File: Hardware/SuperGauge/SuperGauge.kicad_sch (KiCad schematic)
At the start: 20 parts, among them J102 MainConn, Q602 MMBT3906, U103 ATmega16U2, U301 NCV1117ST50T3G

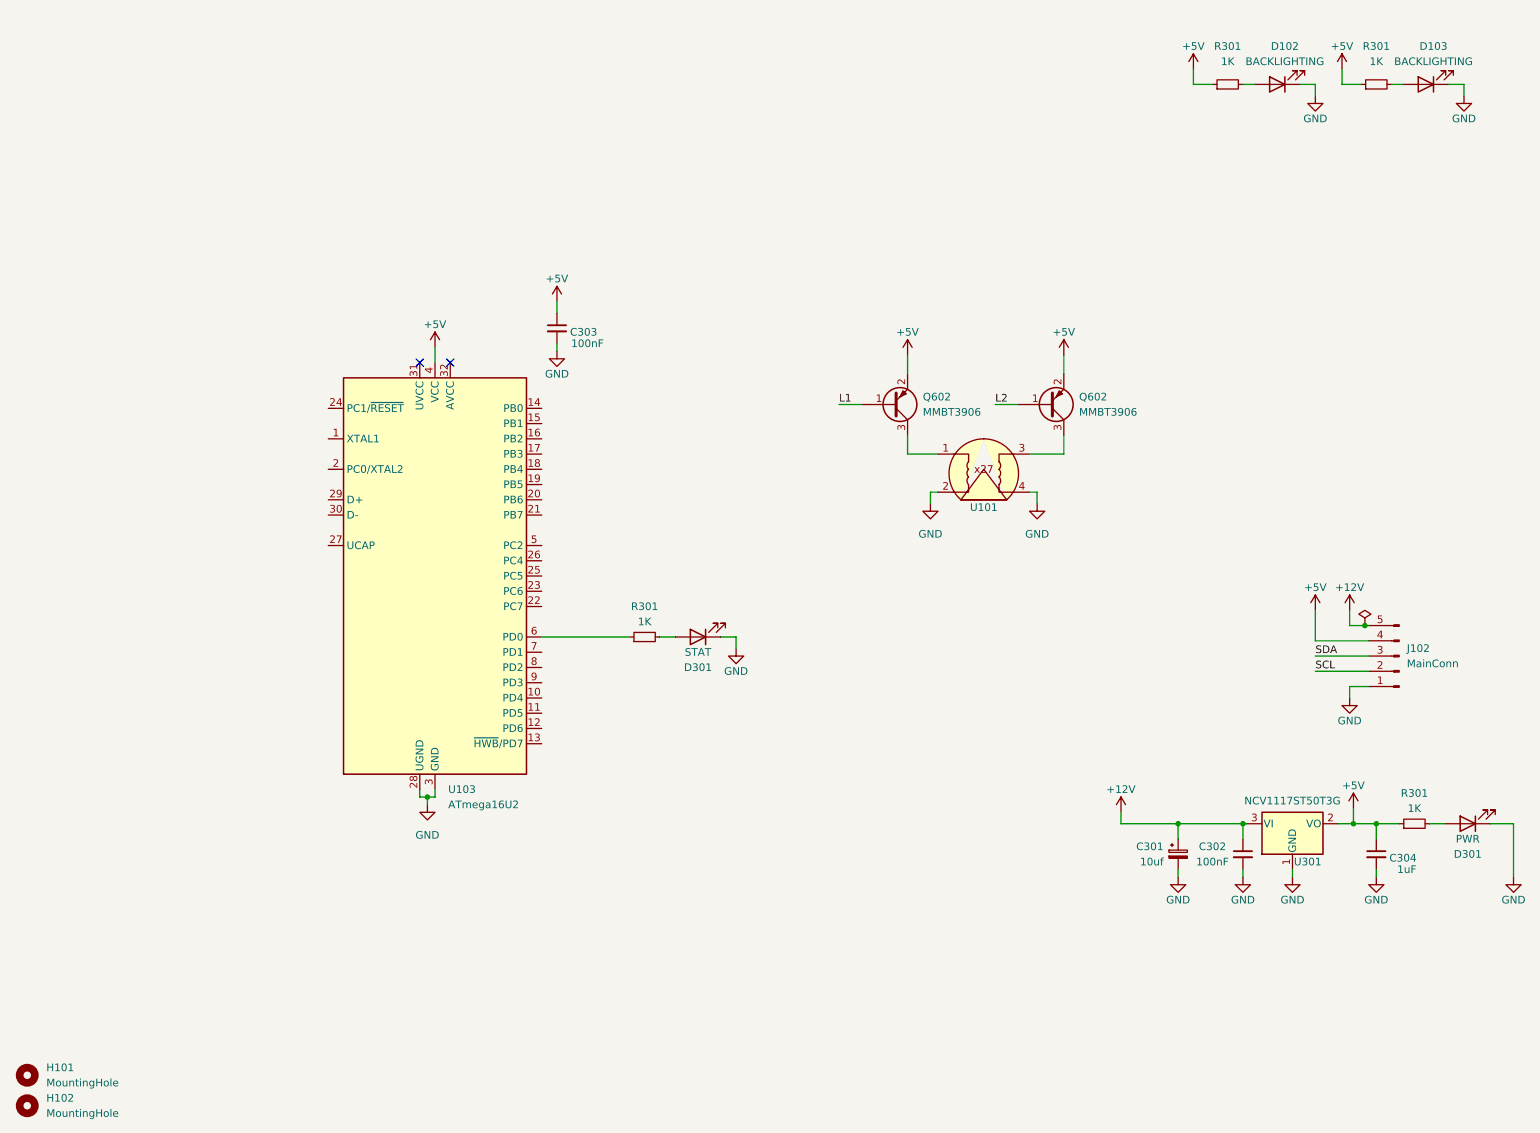
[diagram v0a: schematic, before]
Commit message: More PCB stuff
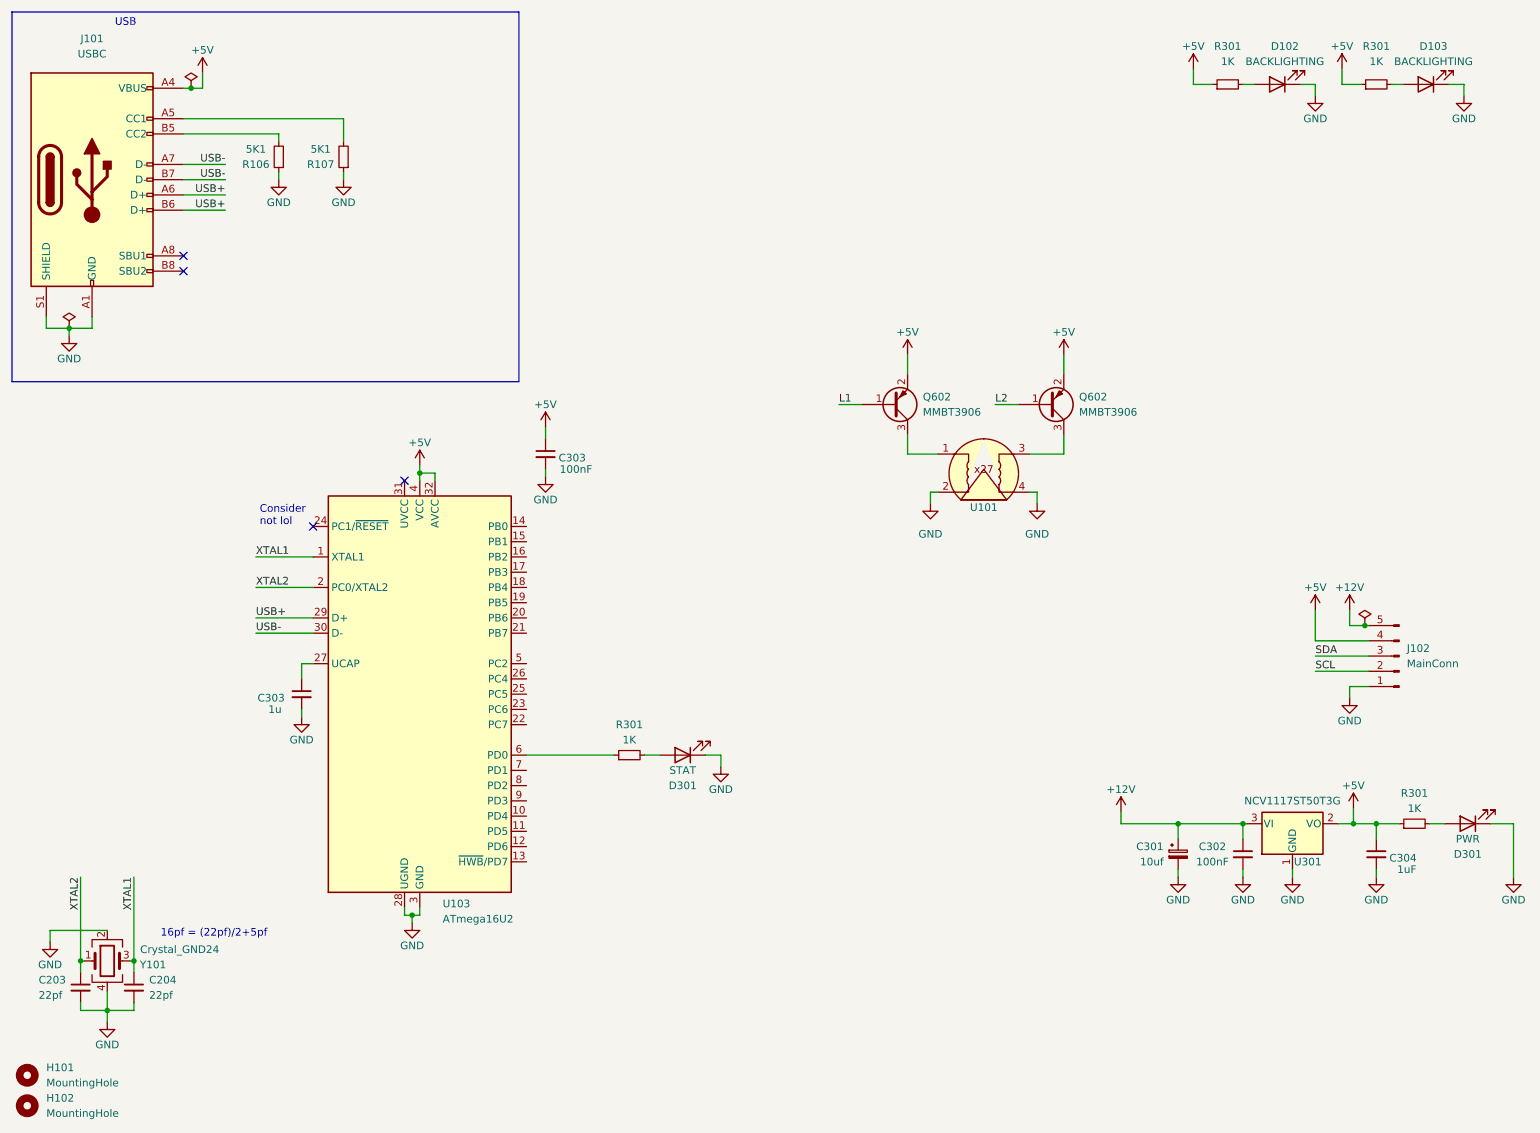
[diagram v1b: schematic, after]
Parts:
- added C203, C204: 22pf, Capacitor_SMD:C_0603_1608Metric, symbol Device:C_Small
- added C303: 1u, Capacitor_SMD:C_0805_2012Metric, symbol Device:C_Small
- added J101: USBC, Connector_USB:USB_C_Receptacle_XKB_U262-16XN-4BVC11, symbol Connector:USB_C_Receptacle_USB2.0
- added R106, R107: 5K1, Resistor_SMD:R_0805_2012Metric, symbol Device:R_Small
- added Y101: Crystal_GND24, Crystal:Crystal_SMD_3225-4Pin_3.2x2.5mm, symbol Device:Crystal_GND24
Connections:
- net +5V: now also U103.32 (AVCC), J101.A4 (VBUS), J101.A9 (VBUS), J101.B4 (VBUS), J101.B9 (VBUS)
- net GND: now also C203.2, C204.2, C303.2, J101.A1 (GND), J101.A12 (GND), J101.B1 (GND), J101.B12 (GND), J101.S1 (SHIELD), R106.1, R107.1, Y101.2, Y101.4
- net XTAL1: now reaches U103.1 (XTAL1)
- net XTAL1: now also C204.1, Y101.3
- net XTAL2: now reaches U103.2 (PC0/XTAL2)
- net XTAL2: now also C203.1, Y101.1
- net at U103.27 (UCAP): now also C303.1
- net USB+: now reaches U103.29 (D+)
- net USB+: now also J101.A6 (D+), J101.B6 (D+)
- net USB-: now reaches U103.30 (D-)
- net USB-: now also J101.A7 (D-), J101.B7 (D-)
- new net: J101.A5 (CC1), R107.2
- new net: J101.B5 (CC2), R106.2
- no-connect marks 2 -> 4
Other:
- note added: "16pf = (22pf)/2+5pf"
- note added: "Consider not lol"
- note added: "USB"
- moved on the sheet: C303, D301, R301, U103
